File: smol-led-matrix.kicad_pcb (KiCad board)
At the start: 4 copper layers, 44.5 x 21.1 mm, 320 parts, among them J1 USB_C_Receptacle_USB2.0, J2 TagConnect_TC2030_SWD, Q1 FS8205, Q2 AO3401A, SW1 SW_Push, SW2 SW_Push, U1 STM32L433CBTx, U2 TP4054, U3 DW01+G, U4 XC6206P332MR

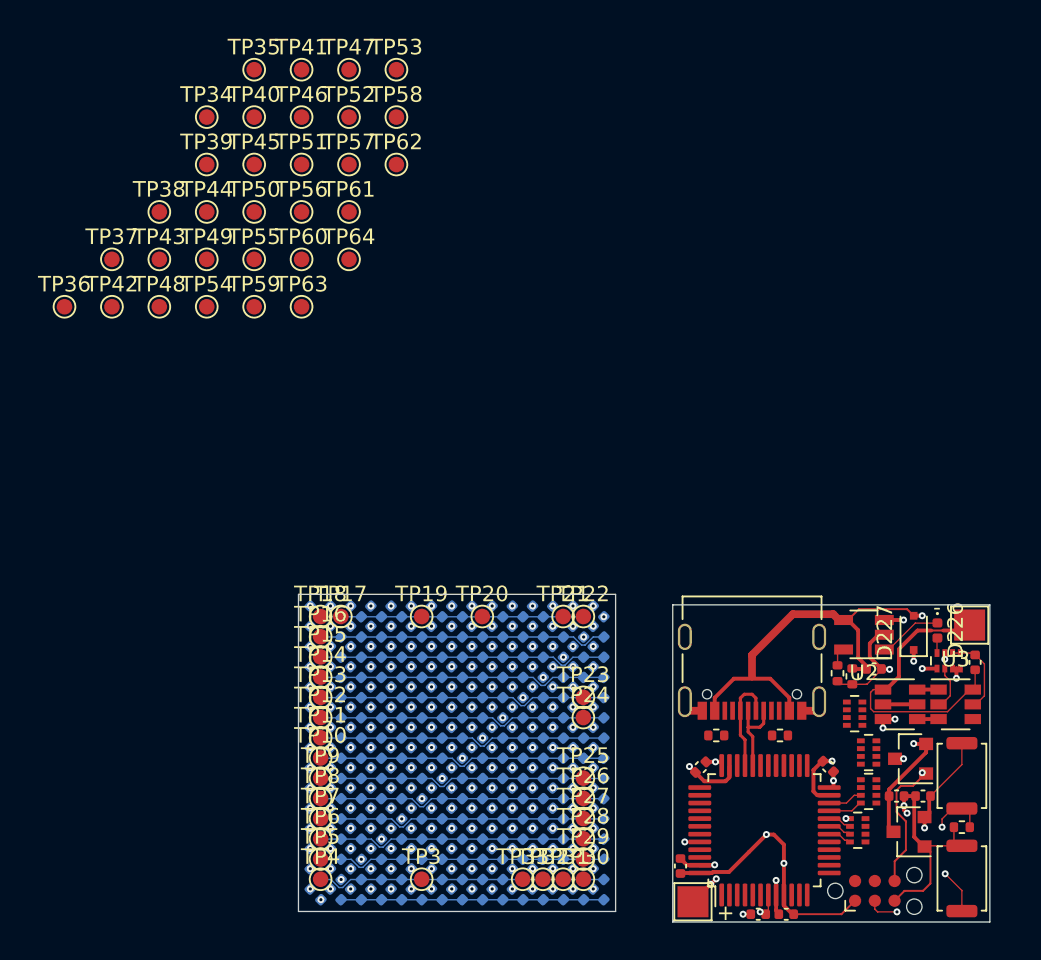
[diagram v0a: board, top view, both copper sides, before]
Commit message: Layout half done
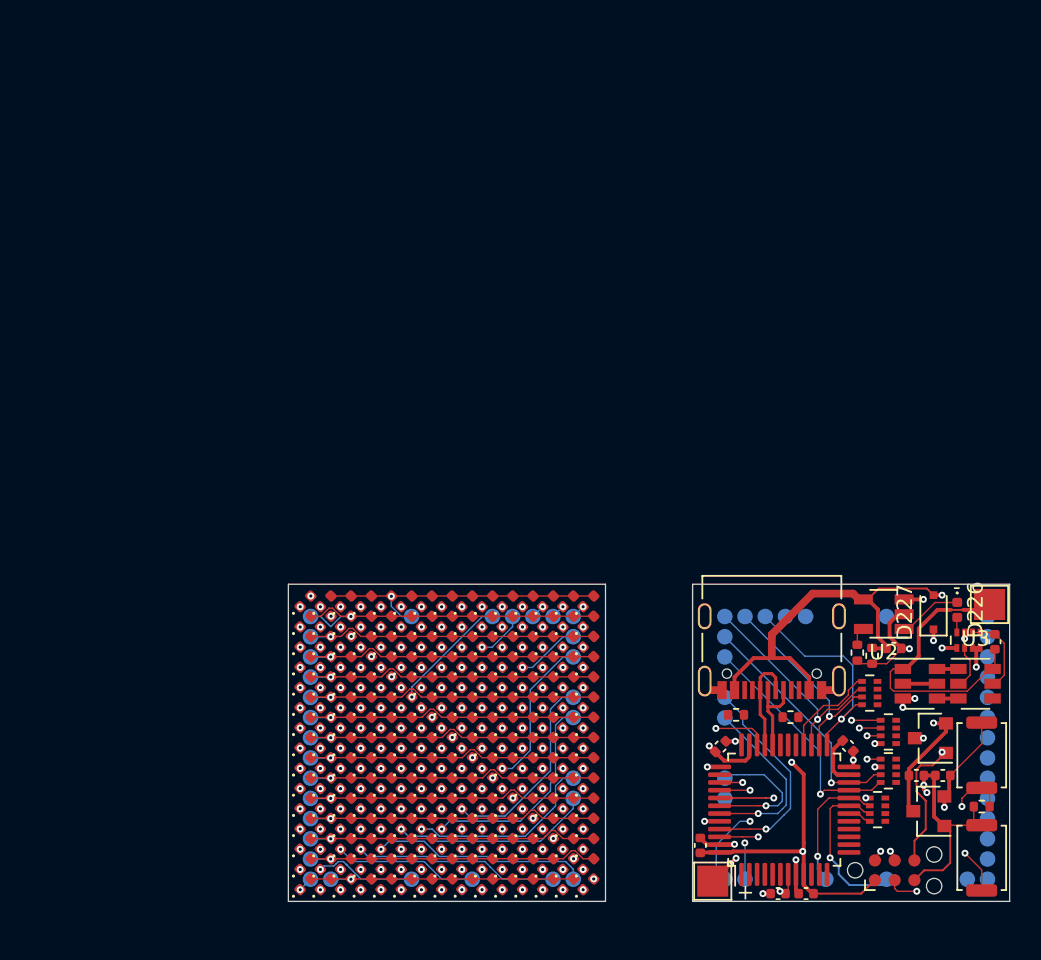
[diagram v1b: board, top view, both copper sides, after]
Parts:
- D1, D10, D100, D101, D102, D103, D104, D105, D106, D107, D108, D109, D11, D110, D111, D112, D113, D114, D115, D116, D117, D118, D119, D12, D120, D121, D122, D123, D124, D125, D126, D127, D128, D129, D13, D130, D131, D132, D133, D134, D135, D136, D137, D138, D139, D14, D140, D141, D142, D143, D144, D145, D146, D147, D148, D149, D15, D150, D151, D152, D153, D154, D155, D156, D157, D158, D159, D16, D160, D161, D162, D163, D164, D165, D166, D167, D168, D169, D17, D170, D171, D172, D173, D174, D175, D176, D177, D178, D179, D18, D180, D181, D182, D183, D184, D185, D186, D187, D188, D189, D19, D190, D191, D192, D193, D194, D195, D196, D197, D198, D199, D2, D20, D200, D201, D202, D203, D204, D205, D206, D207, D208, D209, D21, D210, D211, D212, D213, D214, D215, D216, D217, D218, D219, D22, D220, D221, D222, D223, D224, D225, D23, D24, D25, D26, D27, D28, D29, D3, D30, D31, D32, D33, D34, D35, D36, D37, D38, D39, D4, D40, D41, D42, D43, D44, D45, D46, D47, D48, D49, D5, D50, D51, D52, D53, D54, D55, D56, D57, D58, D59, D6, D60, D61, D62, D63, D64, D65, D66, D67, D68, D69, D7, D70, D71, D72, D73, D74, D75, D76, D77, D78, D79, D8, D80, D81, D82, D83, D84, D85, D86, D87, D88, D89, D9, D90, D91, D92, D93, D94, D95, D96, D97, D98, D99: moved to F.Cu
- TP10, TP11, TP12, TP13, TP14, TP15, TP16, TP17, TP18, TP19, TP20, TP21, TP22, TP23, TP24, TP25, TP26, TP27, TP28, TP29, TP3, TP30, TP31, TP32, TP33, TP34, TP35, TP36, TP37, TP38, TP39, TP4, TP40, TP41, TP42, TP43, TP44, TP45, TP46, TP47, TP48, TP49, TP5, TP50, TP51, TP52, TP53, TP54, TP55, TP56, TP57, TP58, TP59, TP6, TP60, TP61, TP62, TP63, TP64, TP7, TP8, TP9: moved to B.Cu
- moved TP47 65.3 mm to (144.6, 115.2)
- moved TP49 64.1 mm to (144.6, 116.5)
- moved TP46 64.0 mm to (144.6, 114.0)
- moved TP48 63.7 mm to (143.2, 116.5)
- moved TP42 63.4 mm to (144.6, 108.8)
- moved TP45 63.2 mm to (144.6, 112.7)
- moved TP36 63.1 mm to (144.6, 101.0)
- moved TP43 62.9 mm to (144.6, 110.0)
- moved TP44 62.8 mm to (144.6, 111.3)
- moved TP37 61.9 mm to (144.6, 102.2)
- moved TP41 61.6 mm to (144.6, 107.5)
- moved TP38 61.1 mm to (144.6, 103.5)
- moved TP40 61.0 mm to (144.6, 106.2)
- moved TP39 60.8 mm to (144.6, 104.8)
- moved TP50 59.1 mm to (138.1, 116.5)
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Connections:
- RN5 pad 1: /K12 -> /K15
- RN5 pad 2: /K13 -> /K14
- RN5 pad 3: /K14 -> /K13
- RN5 pad 4: Net-(RN5-Pad4) -> /K12
- RN5 pad 5: Net-(RN5-Pad5) -> /A12
- RN5 pad 6: /A14 -> /A13
- RN5 pad 7: /A13 -> /A14
- RN5 pad 8: /A12 -> /A15
- TP33 pad 1: /K15 -> /A15
- TP64 pad 1: /K15 -> /A15
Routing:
- net /K8: track 18.2 -> 54.3 mm, vias 15 -> 17
- net /K7: track 18.2 -> 53.4 mm, vias 15 -> 17
- net /K4: track 18.2 -> 51.6 mm, vias 15 -> 18
- net /K6: track 18.2 -> 48.7 mm, vias 15 -> 17
- net /K3: track 18.5 -> 48.7 mm, vias 16 -> 18
- net /K5: track 18.2 -> 46.4 mm, vias 15 -> 17
- net Net-(J2-Pad2): track 0.00 -> 24.5 mm, vias 0 -> 2
- net /K10: track 20.4 -> 43.6 mm, vias 15 -> 16
- net Net-(J2-Pad4): track 0.00 -> 22.0 mm, vias 0 -> 2
- net /K11: track 20.4 -> 37.9 mm, vias 15 -> 16
- net /K1: track 19.6 -> 35.9 mm, vias 15 -> 16
- net /K2: track 19.6 -> 35.7 mm, vias 15 -> 16
- net /K14: track 18.2 -> 34.2 mm, vias 15 -> 16
- net /K9: track 18.2 -> 33.6 mm, vias 15 -> 17
- net /K12: track 18.2 -> 33.5 mm, vias 15 -> 16
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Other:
- board size 44.5 x 21.1 mm -> 46.4 x 20.4 mm
